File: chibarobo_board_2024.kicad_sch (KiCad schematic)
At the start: 6 parts, among them IC1 ESP32-S2-DevKitM-1, J1 Conn_01x14_Socket

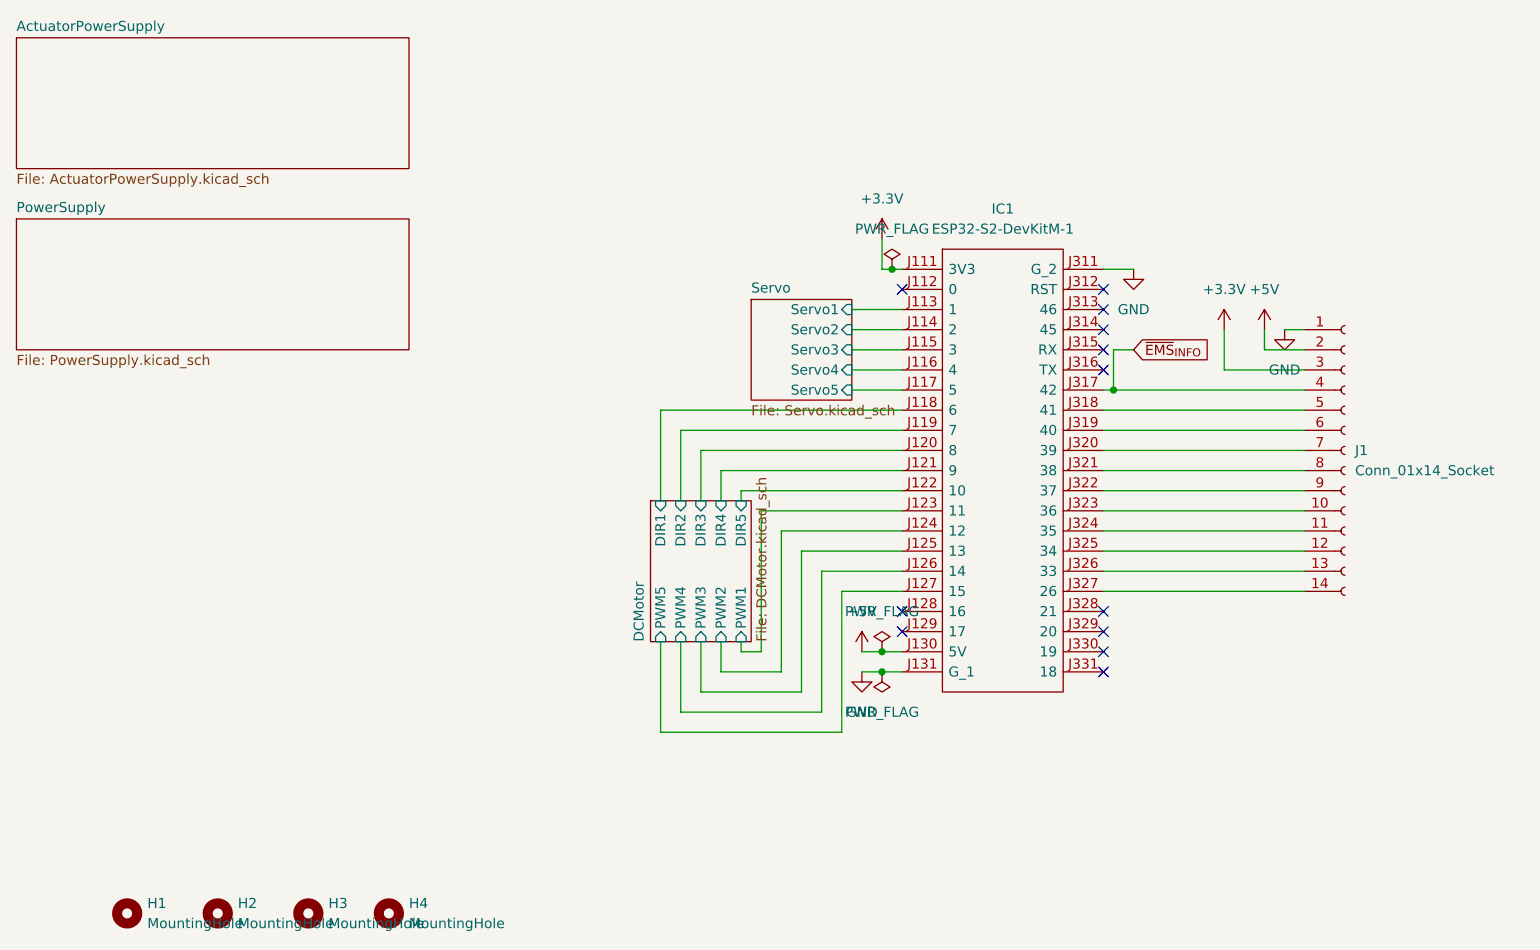
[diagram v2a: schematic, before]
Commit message: Rev2
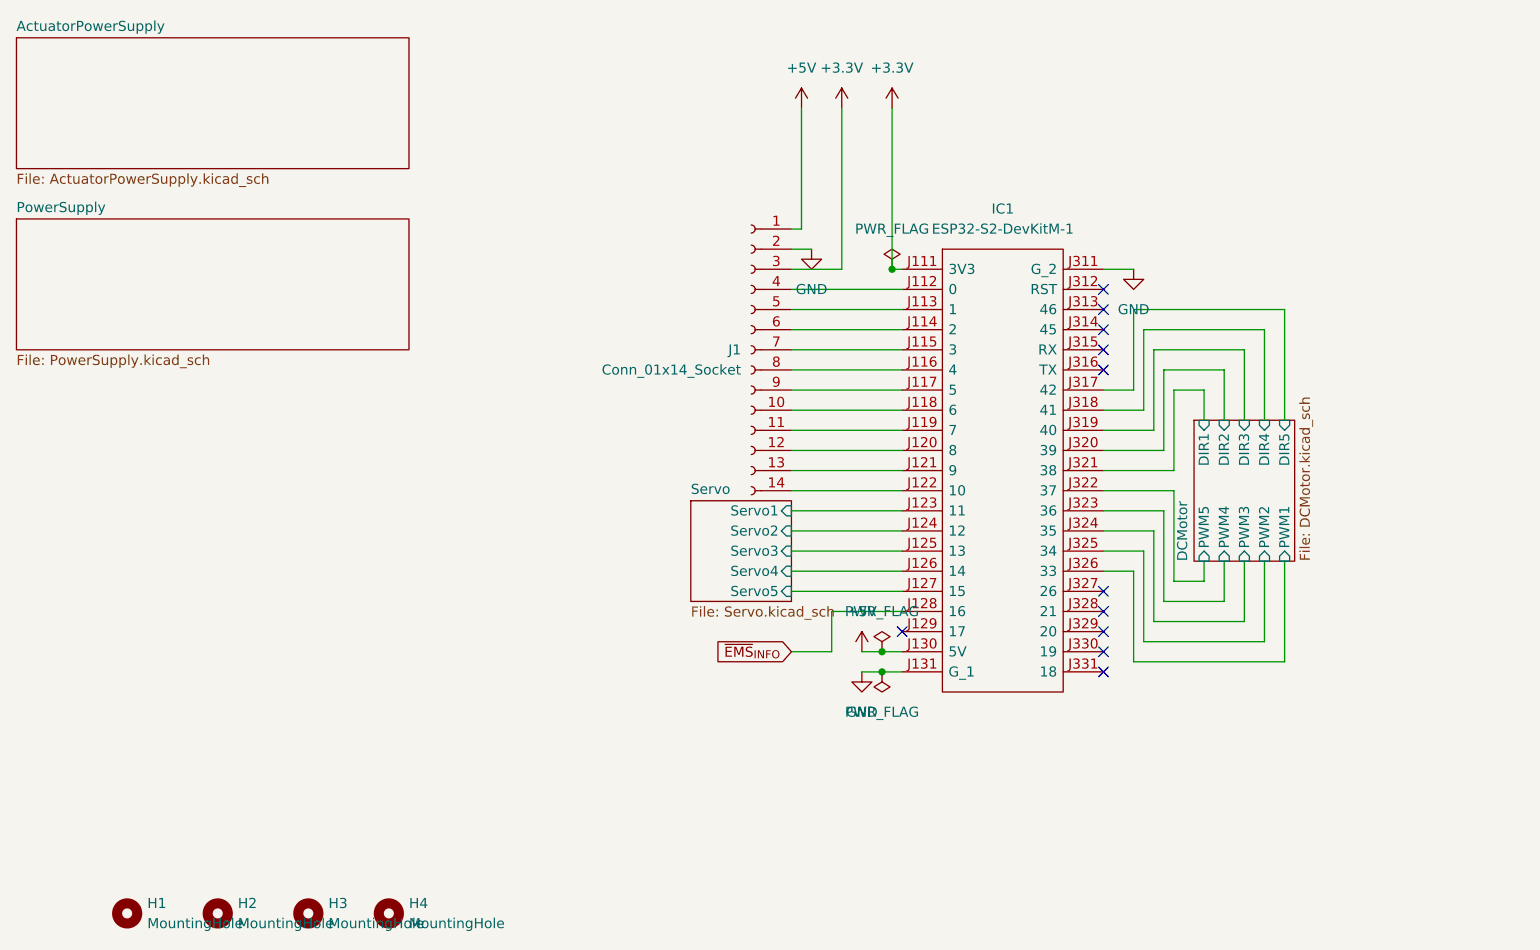
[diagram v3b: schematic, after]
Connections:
- net +5V: now also J1.1 (Pin_1); no longer J1.2 (Pin_2)
- net DCMotor/DIR1: now also IC1.J321 (38); no longer IC1.J118 (6)
- net DCMotor/DIR2: now also IC1.J320 (39); no longer IC1.J119 (7)
- net DCMotor/DIR3: now also IC1.J319 (40); no longer IC1.J120 (8)
- net DCMotor/DIR4: now also IC1.J318 (41); no longer IC1.J121 (9)
- net DCMotor/DIR5: now also IC1.J317 (42); no longer IC1.J122 (10)
- net DCMotor/PWM1: now also IC1.J326 (33); no longer IC1.J123 (11)
- net DCMotor/PWM2: now also IC1.J325 (34); no longer IC1.J124 (12)
- net DCMotor/PWM3: now also IC1.J324 (35); no longer IC1.J125 (13)
- net DCMotor/PWM4: now also IC1.J323 (36); no longer IC1.J126 (14)
- net DCMotor/PWM5: now also IC1.J322 (37); no longer IC1.J127 (15)
- net GND: now also J1.2 (Pin_2); no longer J1.1 (Pin_1)
- net Servo/Servo1: now also IC1.J123 (11); no longer IC1.J113 (1)
- net Servo/Servo2: now also IC1.J124 (12); no longer IC1.J114 (2)
- net Servo/Servo3: now also IC1.J125 (13); no longer IC1.J115 (3)
- net Servo/Servo4: now also IC1.J126 (14); no longer IC1.J116 (4)
- net Servo/Servo5: now also IC1.J127 (15); no longer IC1.J117 (5)
- net ~{EMS}_{INFO}: now also IC1.J128 (16); no longer IC1.J317 (42), J1.4 (Pin_4)
- net at IC1.J112 (0): now also J1.4 (Pin_4)
- net at J1.5 (Pin_5): now also IC1.J113 (1); no longer IC1.J318 (41)
- net at J1.6 (Pin_6): now also IC1.J114 (2); no longer IC1.J319 (40)
- net at J1.7 (Pin_7): now also IC1.J115 (3); no longer IC1.J320 (39)
- net at J1.8 (Pin_8): now also IC1.J116 (4); no longer IC1.J321 (38)
- net at J1.9 (Pin_9): now also IC1.J117 (5); no longer IC1.J322 (37)
- net at J1.10 (Pin_10): now also IC1.J118 (6); no longer IC1.J323 (36)
- net at J1.11 (Pin_11): now also IC1.J119 (7); no longer IC1.J324 (35)
- net at J1.12 (Pin_12): now also IC1.J120 (8); no longer IC1.J325 (34)
- net at J1.13 (Pin_13): now also IC1.J121 (9); no longer IC1.J326 (33)
- net at J1.14 (Pin_14): now also IC1.J122 (10); no longer IC1.J327 (26)
- no-connect marks 12 -> 11
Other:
- moved on the sheet: J1
